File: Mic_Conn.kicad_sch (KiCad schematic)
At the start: 5 parts, among them J6 JST_SH_1x4_SM04B-SRSS-TB-LF-SN, U1 TPD4E05U06QDQARQ1

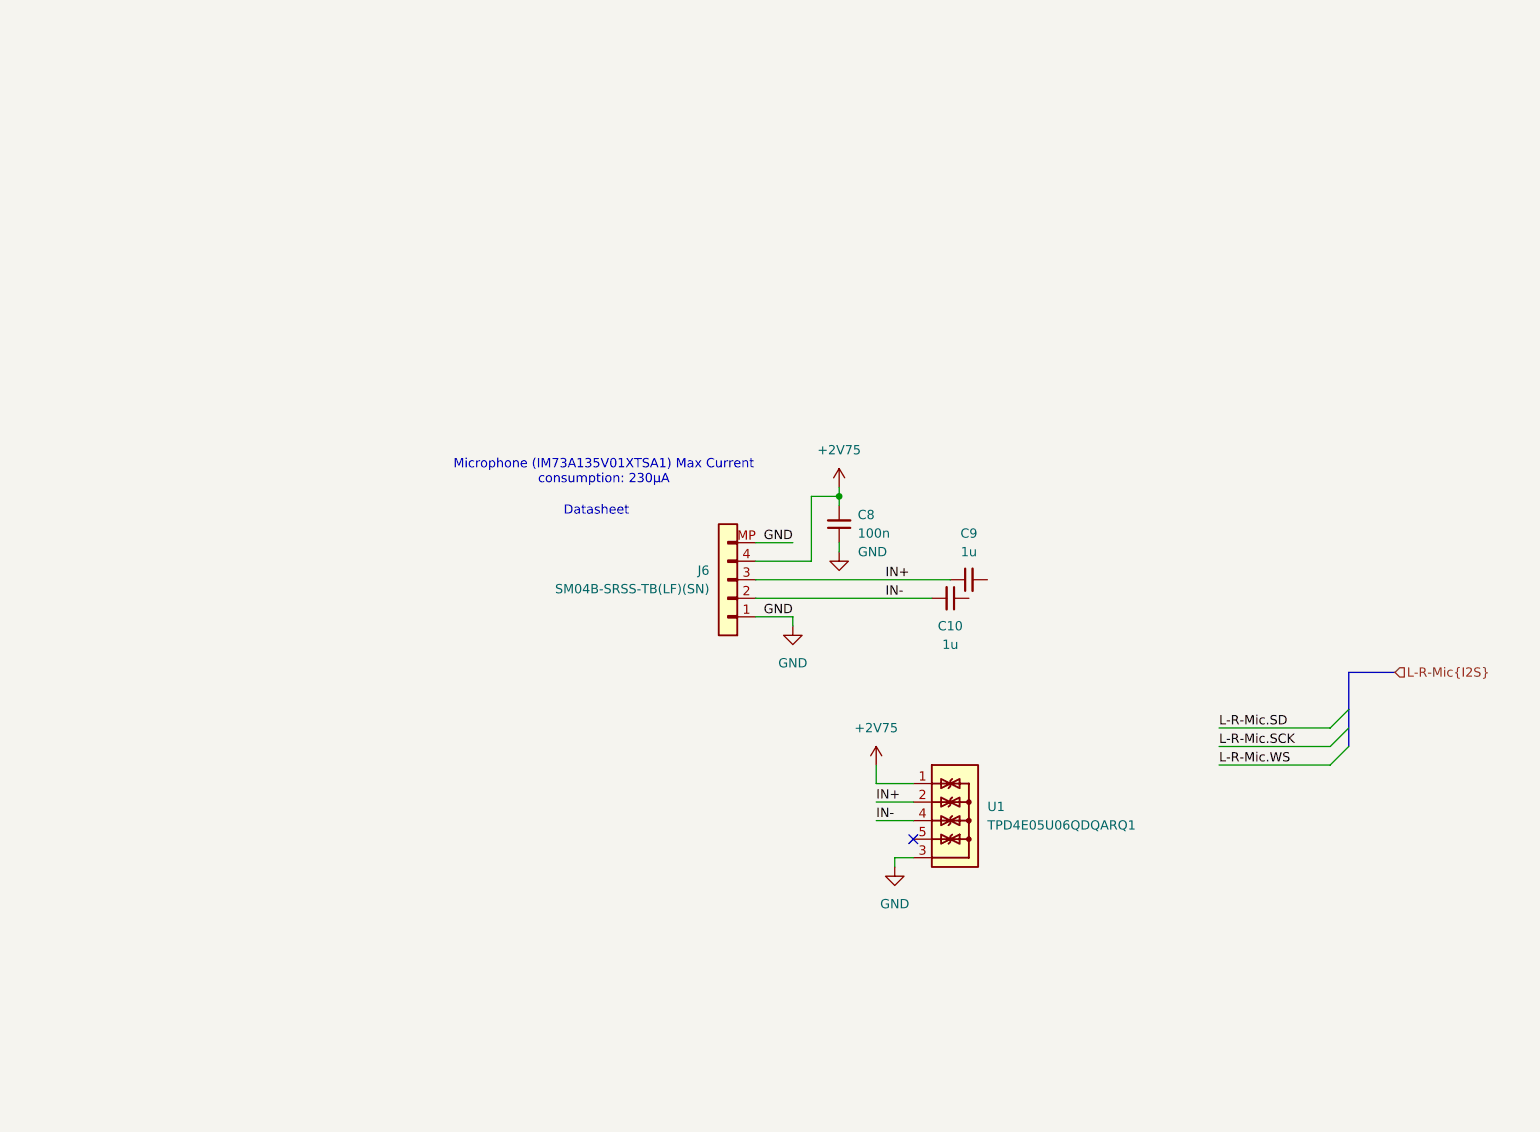
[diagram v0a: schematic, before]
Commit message: [#71555] Draw MIC and USB Connector sheets
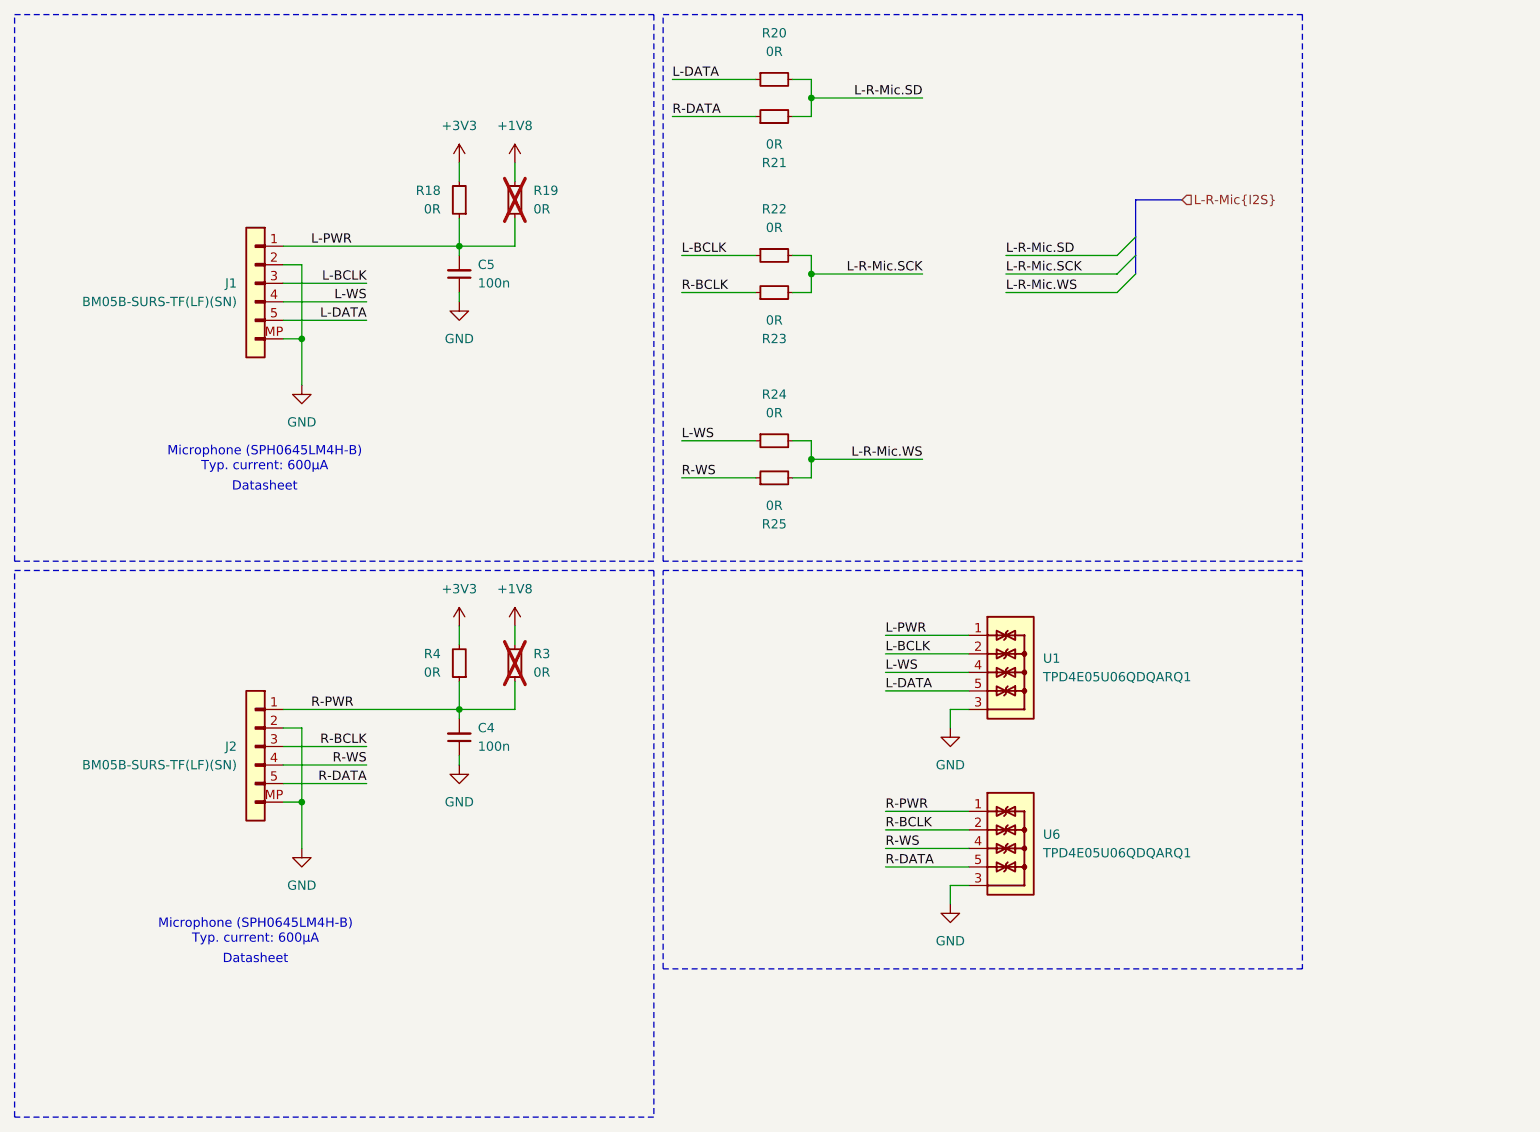
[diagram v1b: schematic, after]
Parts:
- removed C10, C9: C_1u_0402, antmicro-footprints:C_0402_1005Metric, symbol antmicroCapacitors0402:C_1u_0402
- removed C8: C_100n_0402, antmicro-footprints:C_0402_1005Metric, symbol antmicroCapacitors0402:C_100n_0402
- removed J6: JST_SH_1x4_SM04B-SRSS-TB-LF-SN, antmicro-footprints:Conn_JST_SH_1x4_SM04B-SRSS-TB-LF-SN, symbol antmicroWire2BoardConnectors:JST_SH_1x4_SM04B-SRSS-TB-LF-SN
- added C4, C5: C_100n_0402, antmicro-footprints:C_0402_1005Metric, symbol antmicroCapacitors0402:C_100n_0402
- added J1, J2: JST_SUR_1x5_BM05B-SURS-TB-LF-SN, antmicro-footprints:Conn_JST_SUR_1x5_BM05B-SURS-TF-LF-SN, symbol antmicroWire2BoardConnectors:JST_SUR_1x5_BM05B-SURS-TB-LF-SN
- added R18, R19, R20, R21, R22, R23, R24, R25, R3, R4: R_0R_0402, antmicro-footprints:R_0402_1005Metric, symbol antmicroResistors0402:R_0R_0402
- added U6: TPD4E05U06QDQARQ1, antmicro-footprints:USON-10_2.5x1mm_P0.5mm, symbol antmicroTVSDiodes:TPD4E05U06QDQARQ1
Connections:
- net GND: now also C4.1, C5.1, J1.2, J1.MP, J2.2, J2.MP, U6.3, U6.8
- net L-R-Mic.SCK: now also R22.2, R23.2
- net L-R-Mic.SD: now also R20.2, R21.2
- net L-R-Mic.WS: now also R24.2, R25.2
- net L-DATA: now reaches U1.5, U1.6
- net L-DATA: now also J1.5, R20.1
- net +2V75 renamed L-PWR
- net L-PWR: now also C5.2, J1.1, R18.1, R19.1
- net IN+ renamed L-BCLK
- net L-BCLK: now also J1.3, R22.1
- net IN- renamed L-WS
- net L-WS: now also J1.4, R24.1
- new net +1V8: R19.2, R3.2
- new net +3V3: R18.2, R4.2
- new net R-BCLK: J2.3, R23.1, U6.2, U6.9
- new net R-DATA: J2.5, R21.1, U6.5, U6.6
- new net R-PWR: C4.2, J2.1, R3.1, R4.1, U6.1, U6.10
- new net R-WS: J2.4, R25.1, U6.4, U6.7
- no-connect marks 1 -> 0
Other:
- note added: "Microphone (SPH0645LM4H-B) Typ. current: 600µA"
- note removed: "Microphone (IM73A135V01XTSA1) Max Current consumption: 230µA"
